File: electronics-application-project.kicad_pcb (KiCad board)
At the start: 2 copper layers, 65 x 51.5 mm, 53 parts, among them J1 Conn_02x03_Odd_Even, J2 Conn_01x02_Pin, J3 Conn_01x02_Pin, J4 Conn_01x02_Pin, U1 W5500, U2 ARJM11C7-114-BA-EW2, U3 LM2574-3.3YN, U4 ATTINY85-20SU, U5 74HC00, Y2 ABLS7M2-25.000MHZ-D-2Y-T

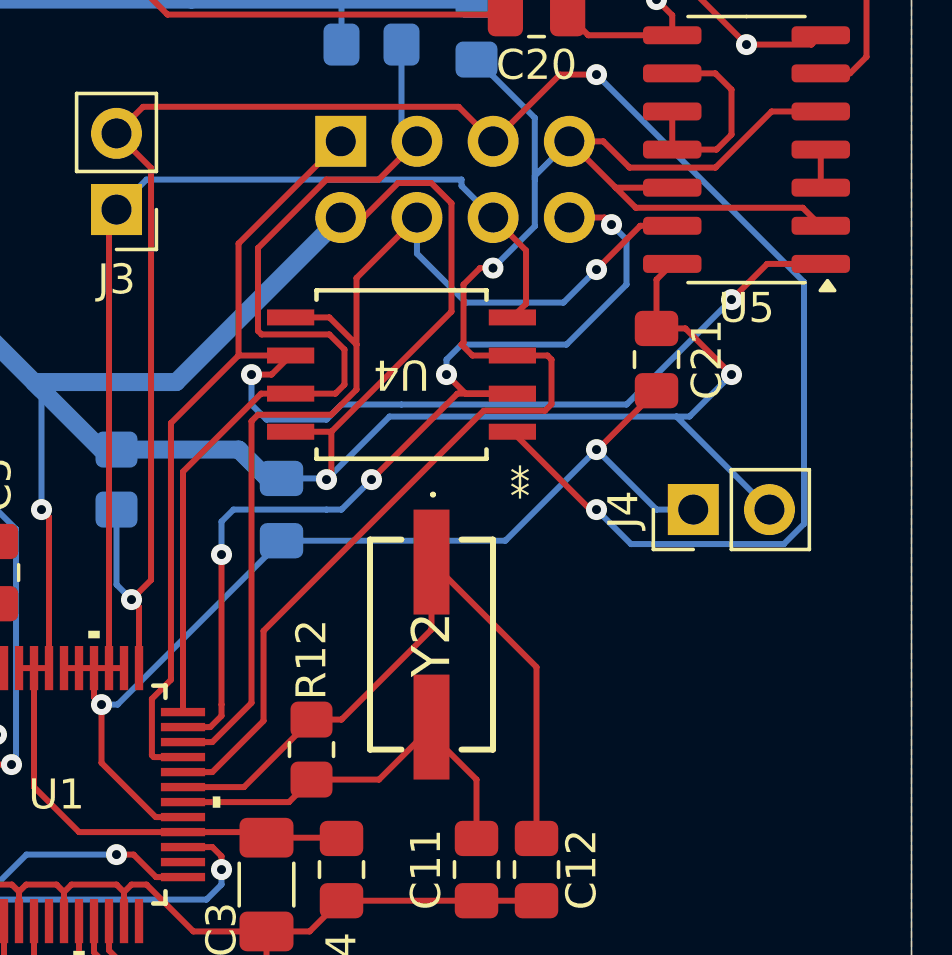
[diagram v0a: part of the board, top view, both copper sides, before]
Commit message: DRC pass
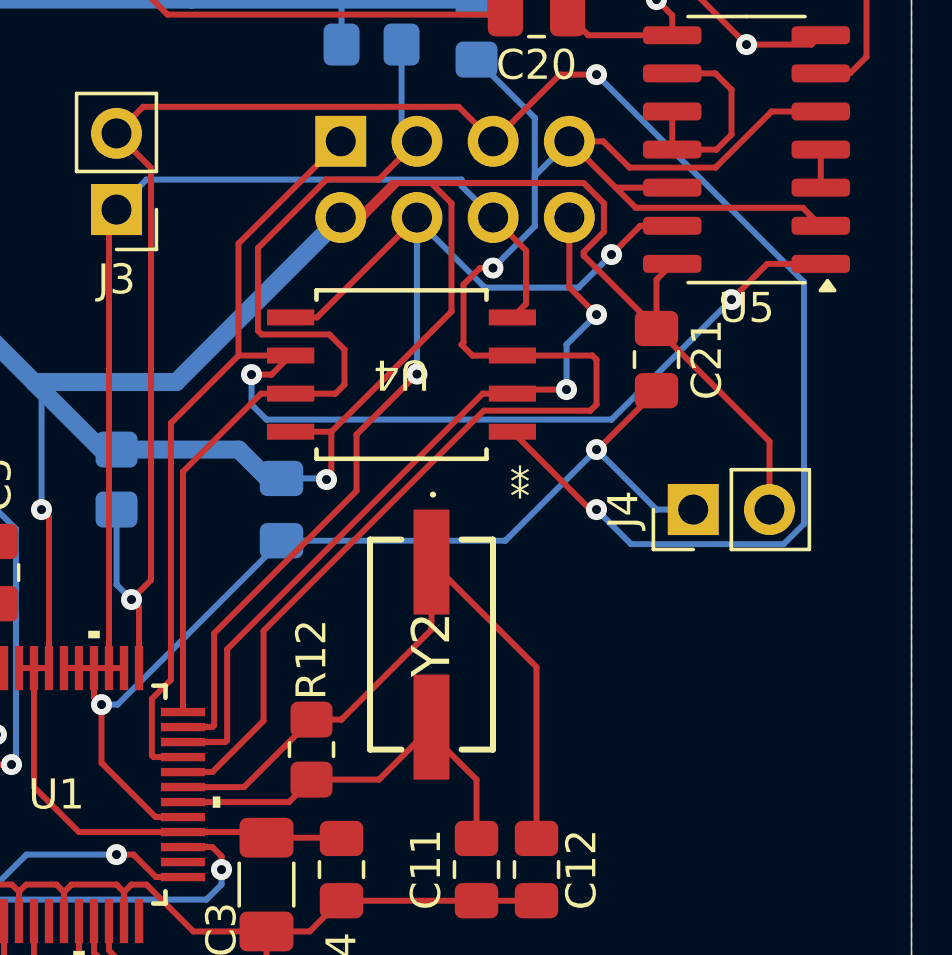
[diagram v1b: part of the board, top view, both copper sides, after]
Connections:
- J1 pad 4: /MISO -> /MOSI
- J1 pad 8: /MOSI -> /MISO
- U4 pad 2: /MOSI -> /MISO
- U4 pad 5: /MISO -> /MOSI
- U5 pad 13: /MISO -> /MOSI
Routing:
- net /MISO: track 36.7 -> 26.5 mm, vias 1 -> 2
- net /MOSI: track 33.1 -> 36.8 mm, vias 4 -> 2
- net /SCSn: track 58.1 -> 61.1 mm
- net 3.3V_D: track 196.7 -> 196.9 mm, vias 3 -> 2
